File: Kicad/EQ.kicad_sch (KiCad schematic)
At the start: 30 parts, among them U5 OPA1656ID

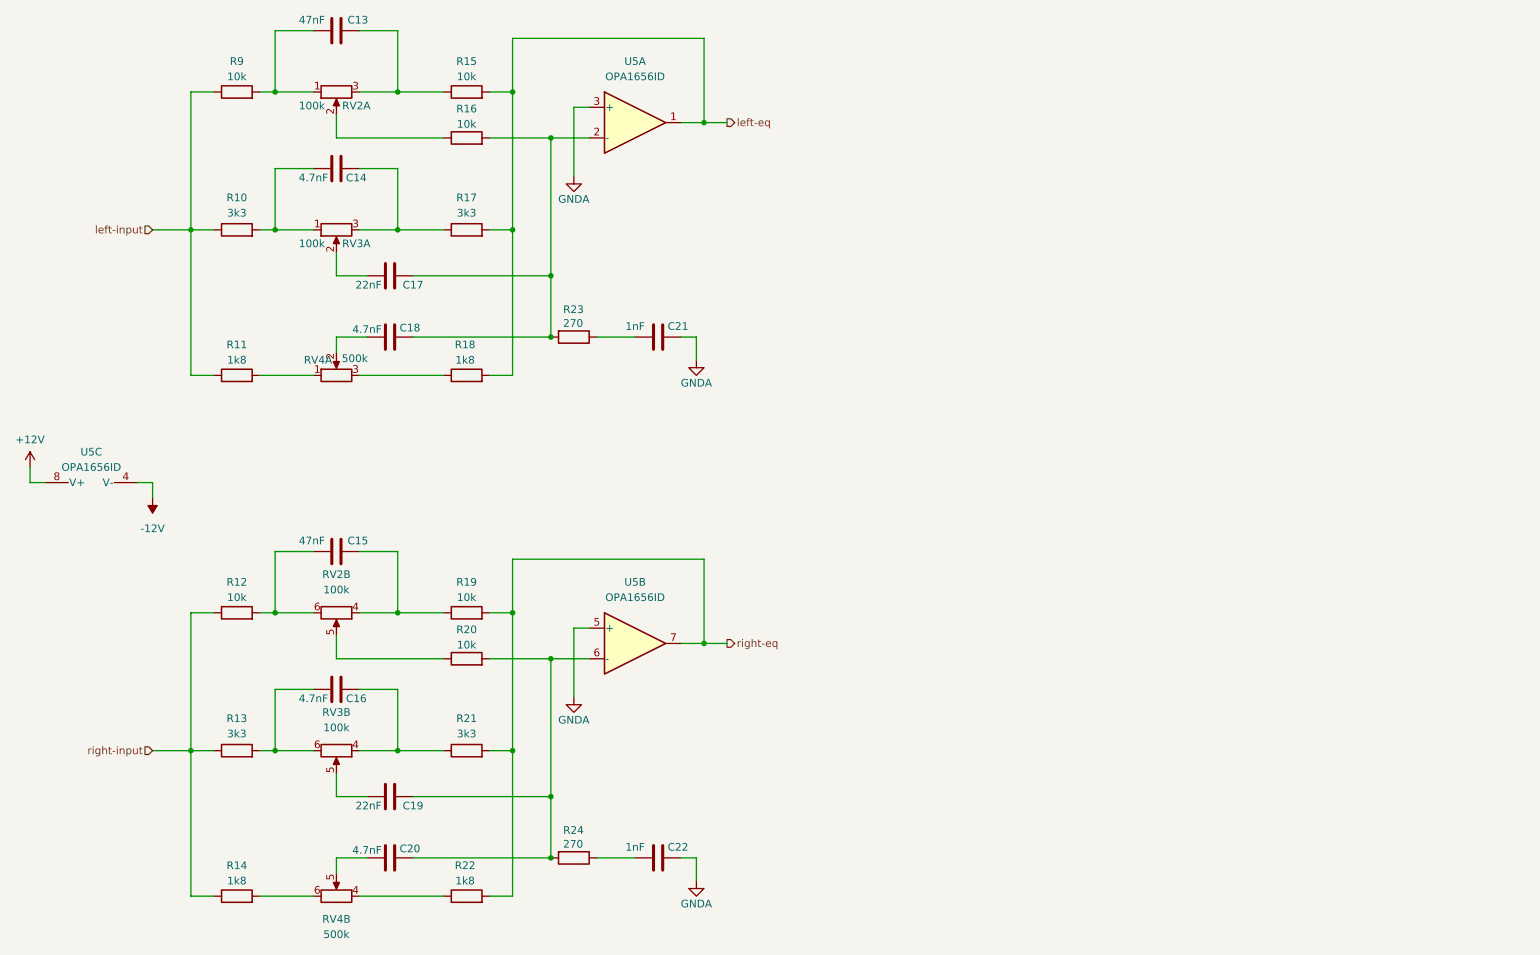
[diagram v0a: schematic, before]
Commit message: final schematic
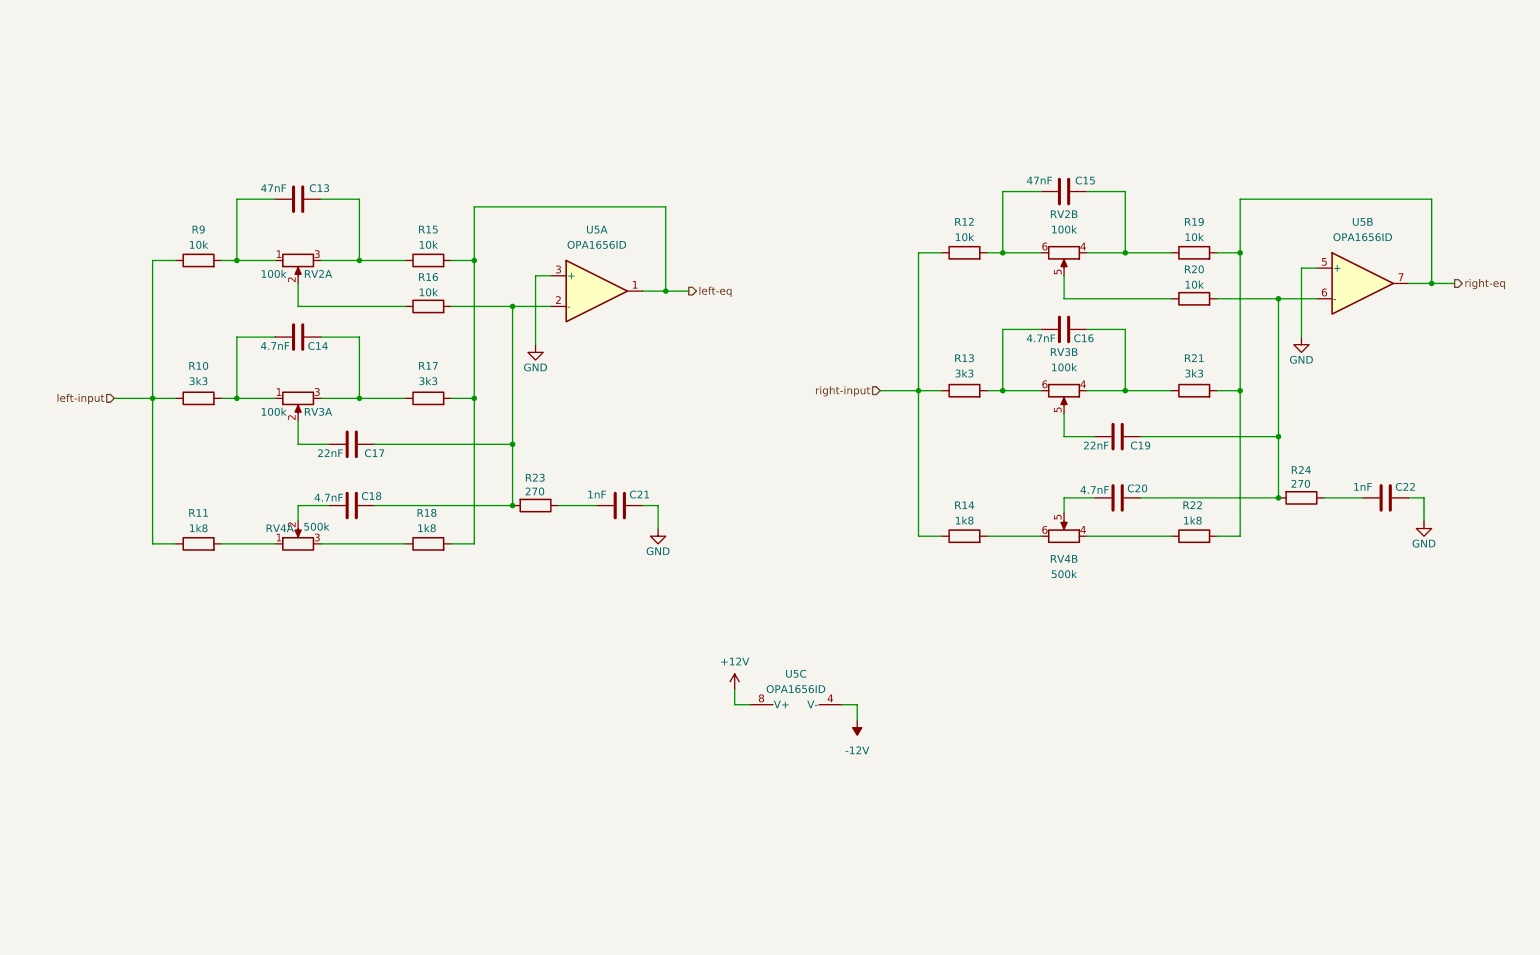
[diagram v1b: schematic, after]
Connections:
- net GNDA renamed GND
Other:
- moved on the sheet: C13, C14, C15, C16, C17, C18, C19, C20, C21, C22, R10, R11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
